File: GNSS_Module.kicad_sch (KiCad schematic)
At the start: 24 parts, among them J2 FTDI_Conn, J4 GPS_Conn, J5 GPS_Conn, J7 LORA_Conn, U11 ublox_SAM-M8Q

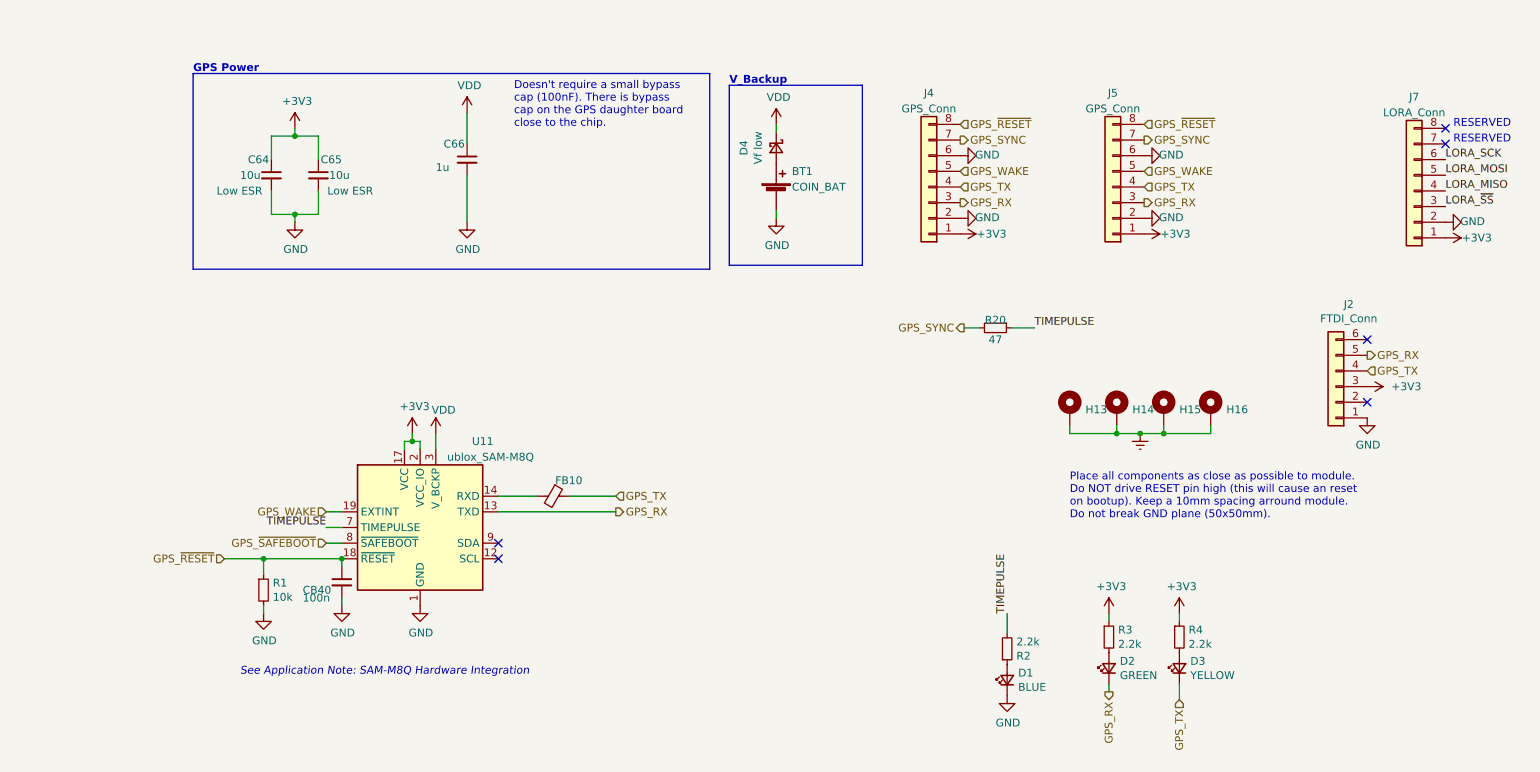
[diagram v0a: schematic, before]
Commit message: big commit
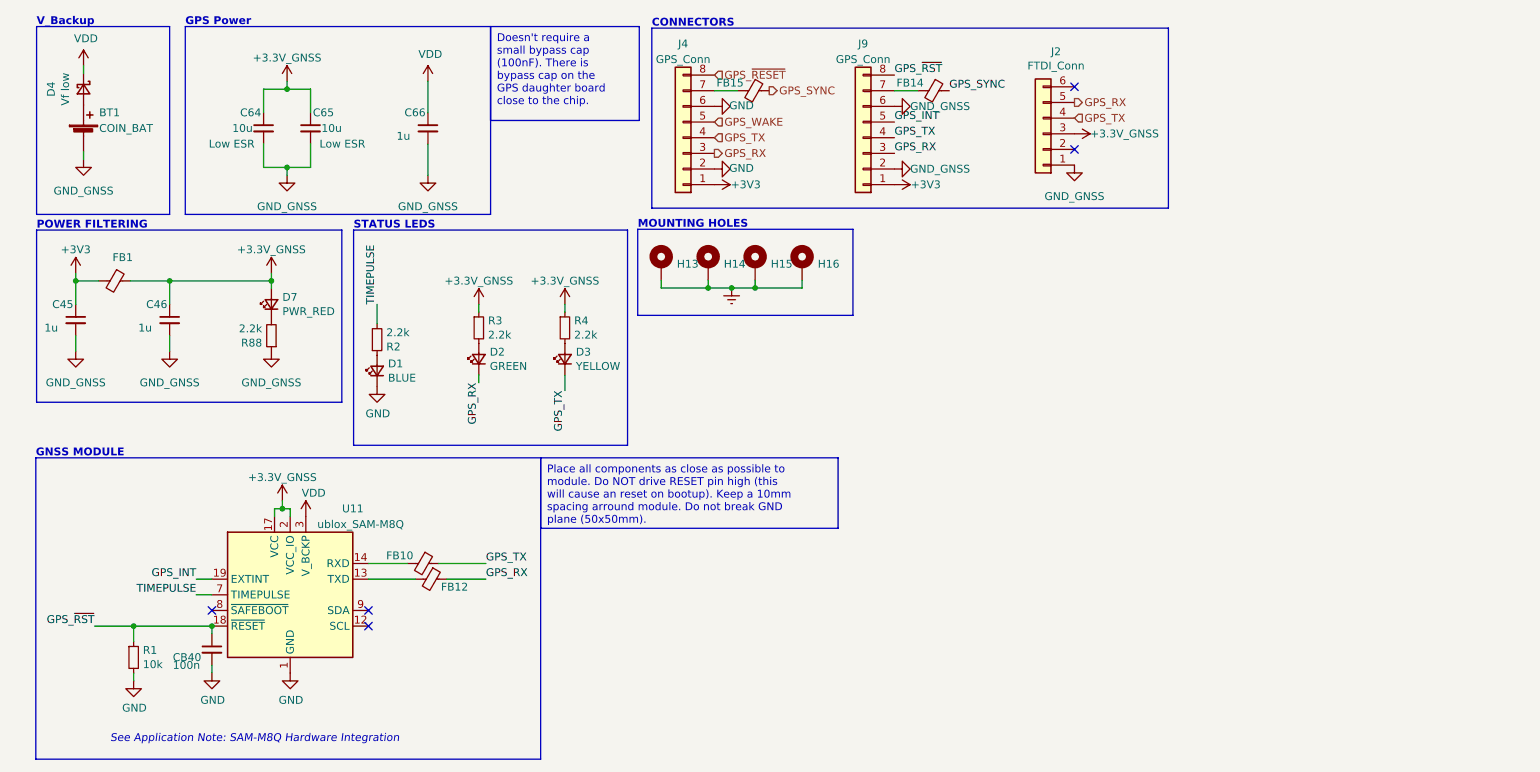
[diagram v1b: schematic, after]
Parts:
- removed J5: GPS_Conn, grootvoet:Connector_Amphenol_10114828-xxx08LF_Vertical, symbol Connector_Generic:Conn_01x08
- removed J7: LORA_Conn, grootvoet:Connector_Amphenol_10114828-xxx08LF_Vertical, symbol Connector_Generic:Conn_01x08
- removed R20: 47, Resistor_SMD:R_0603_1608Metric_Pad0.98x0.95mm_HandSolder, symbol Device:R_Small
- added C45, C46: 1u, Capacitor_SMD:C_0603_1608Metric_Pad1.08x0.95mm_HandSolder, symbol Device:C_Small
- added D7: PWR_RED, LED_SMD:LED_0603_1608Metric_Pad1.05x0.95mm_HandSolder, symbol Device:LED_Small
- added FB1: BLM18KG101TZ1D, Inductor_SMD:L_0603_1608Metric_Pad1.05x0.95mm_HandSolder, symbol Device:Ferrite_Bead_Small
- added FB12, FB14, FB15: BLM15HD102SN1, Inductor_SMD:L_0402_1005Metric, symbol Device:Ferrite_Bead_Small
- added J9: GPS_Conn, grootvoet:Connector_Amphenol_10114828-xxx08LF_Vertical, symbol Connector_Generic:Conn_01x08
- added R88: 2.2k, Resistor_SMD:R_0603_1608Metric_Pad0.98x0.95mm_HandSolder, symbol Device:R_Small
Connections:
- net +3V3: now also C45.1, FB1.2, J9.1 (Pin_1); no longer C64.1, C65.1, J2.3 (Pin_3), R3.1, R4.1, U11.17 (VCC), U11.2 (VCC_IO)
- net GND: now also C45.2, C46.2, J9.2 (Pin_2), J9.6 (Pin_6), R88.1
- net GPS_RX: now also FB12.1, J9.3 (Pin_3); no longer U11.13 (TXD)
- net GPS_SYNC: now also FB14.1, FB15.1; no longer J4.7 (Pin_7)
- net GPS_TX: now also J9.4 (Pin_4)
- net GPS_WAKE: no longer U11.19 (EXTINT)
- net GPS_~{RESET}: no longer CB40.1, R1.1, U11.18 (~{RESET})
- net GPS_~{SAFEBOOT}: no longer names the net of U11.8 (~{SAFEBOOT})
- new net: FB12.2, U11.13 (TXD)
- new net: FB15.2, J4.7 (Pin_7)
- new net: D7.1 (K), R88.2
- new net: FB14.2, J9.7 (Pin_7)
- new net +3.3V: C46.1, C64.1, C65.1, D7.2 (A), FB1.1, J2.3 (Pin_3), R3.1, R4.1, U11.17 (VCC), U11.2 (VCC_IO)
- new net GPS_INT: J9.5 (Pin_5), U11.19 (EXTINT)
- new net GPS_~{RST}: CB40.1, J9.8 (Pin_8), R1.1, U11.18 (~{RESET})
- no-connect marks 6 -> 5
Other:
- note added: "CONNECTORS"
- note added: "GNSS MODULE"
- note added: "MOUNTING HOLES"
- note added: "POWER FILTERING"
- note added: "STATUS LEDS"
- note removed: "Doesn't require a small bypass cap (100nF). There is bypass cap on the GPS daughter board close to the chip."
- note removed: "Place all components as close as possible to module. Do NOT drive RESET pin high (this will cause an reset on bootup). Keep a 10mm spacing arround module. Do not break GND plane (50x50mm)."
- note removed: "RESERVED"
- moved on the sheet: BT1, C64, C65, C66, CB40, D1, D2, D3, D4, FB10, H13, H14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
